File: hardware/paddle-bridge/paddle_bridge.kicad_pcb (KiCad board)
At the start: 2 copper layers, 47.5 x 40 mm, 15 parts, among them J1 APOLLO (P4 header GND,52,51,5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, J2 MACHINE: paddle pair + Micra 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, U1 AQY212EH, U2 LH1502BB, U3 LH1502BB

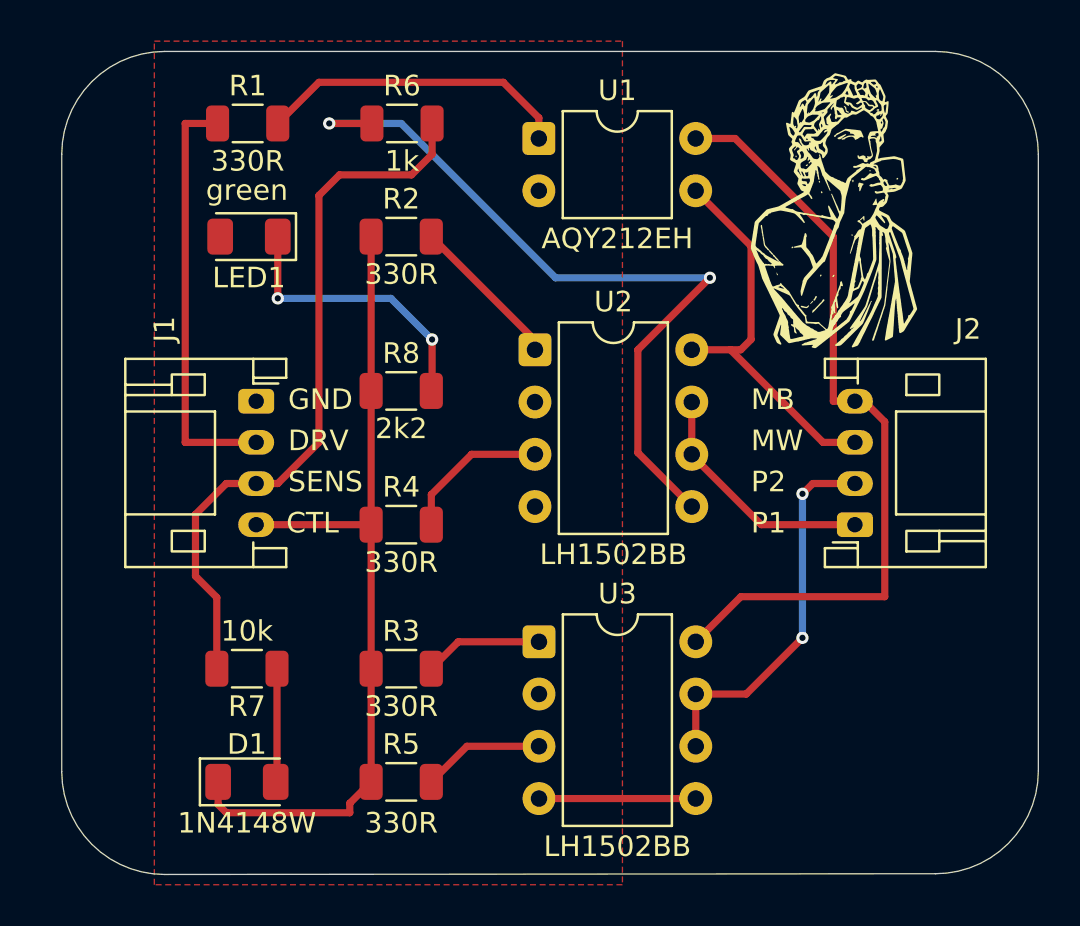
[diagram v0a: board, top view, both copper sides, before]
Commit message: hardware: Apollo Link board update; gerber zip regenerated
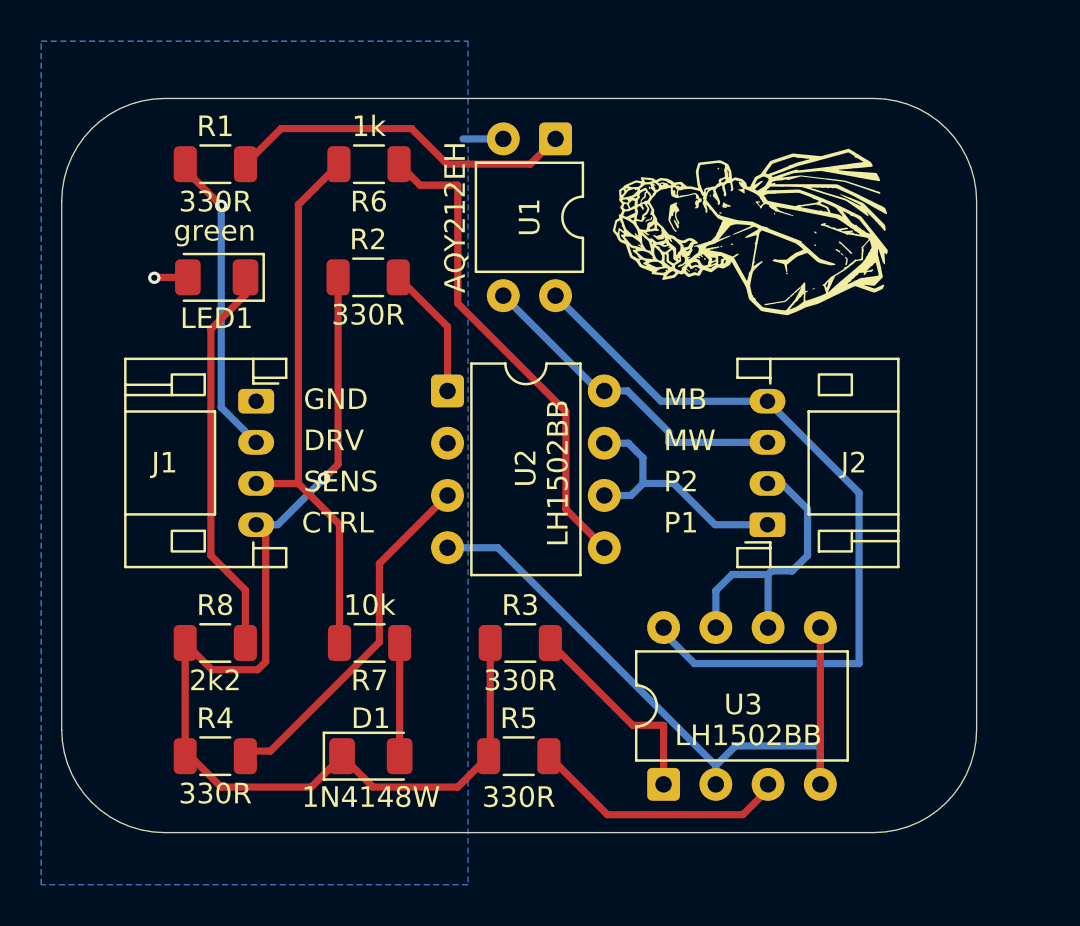
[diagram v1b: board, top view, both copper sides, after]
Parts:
- J2: value MACHINE: paddle pair + Micra white/black -> MACHINE: paddle + Micra white/black
- moved R8 15.2 mm to (126.0, 88.8)
- moved R4 14.4 mm to (126.0, 94.2)
- moved U3 9.20 mm to (147.8, 95.6), turned to 90 degrees
- moved D1 6.15 mm to (133.5, 94.2)
- moved R7 6.09 mm to (133.5, 88.8)
- moved R3 5.92 mm to (140.8, 88.8)
- moved R5 5.85 mm to (140.7, 94.2)
- moved U2 4.70 mm to (137.2, 76.5)
- moved J2 4.25 mm to (152.8, 83.0)
- moved R2 2.55 mm to (133.4, 71.0)
- moved R6 2.55 mm to (133.4, 65.5), turned to 180 degrees
- moved LED1 2.53 mm to (126.0, 71.0)
- moved R1 2.53 mm to (126.0, 65.5)
- moved U1 0.81 mm to (142.5, 64.2), turned to -90 degrees
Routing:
- net /GND_R: track 7.62 -> 37.3 mm, vias 0 -> 1
- net /SENSE_RAW: track 37.3 -> 23.8 mm, vias 2 -> 0
- net /CTRL: track 41.7 -> 53.9 mm, vias 0 -> 1
- net Net-(U2-A2): track 7.31 -> 17.2 mm
- net /SENSE: track 35.2 -> 27.0 mm
- net Net-(U3-A2): track 5.95 -> 12.3 mm
- net /DRIVE: track 20.5 -> 14.9 mm, vias 0 -> 1
- net Net-(LED1-A): track 13.8 -> 19.2 mm, vias 2 -> 0
- net Net-(U3-A1): track 5.78 -> 10.3 mm
- net /P2: track 18.6 -> 14.8 mm, vias 2 -> 0
- net /MICRA_W: track 19.3 -> 16.1 mm
- net Net-(U1-A): track 15.2 -> 17.0 mm
- net Net-(U2-A1): track 7.59 -> 6.51 mm
- net /MICRA_B: track 38.2 -> 37.1 mm
- net /P1: track 11.9 -> 12.4 mm
- added copper zone on B.Cu, net /GND_R
- removed copper zone on F.Cu, net /GND_R
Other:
- board size 47.5 x 40 mm -> 44.5 x 35.7 mm
- board text added: "CTRL"
- board text removed: "CTL"
